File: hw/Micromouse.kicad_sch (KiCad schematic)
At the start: 19 parts, among them J1 MOTOR_LEFT, J2 MOTOR_RIGHT, J3 ENCODER_LEFT, J4 ENCODER_RIGHT, J5 LIDAR_360, SW1 Power Switch, U1 LM2596 - 5V, U2 MP1584EN Buck 3V3, U3 ESP32-C3-DevKitM-1

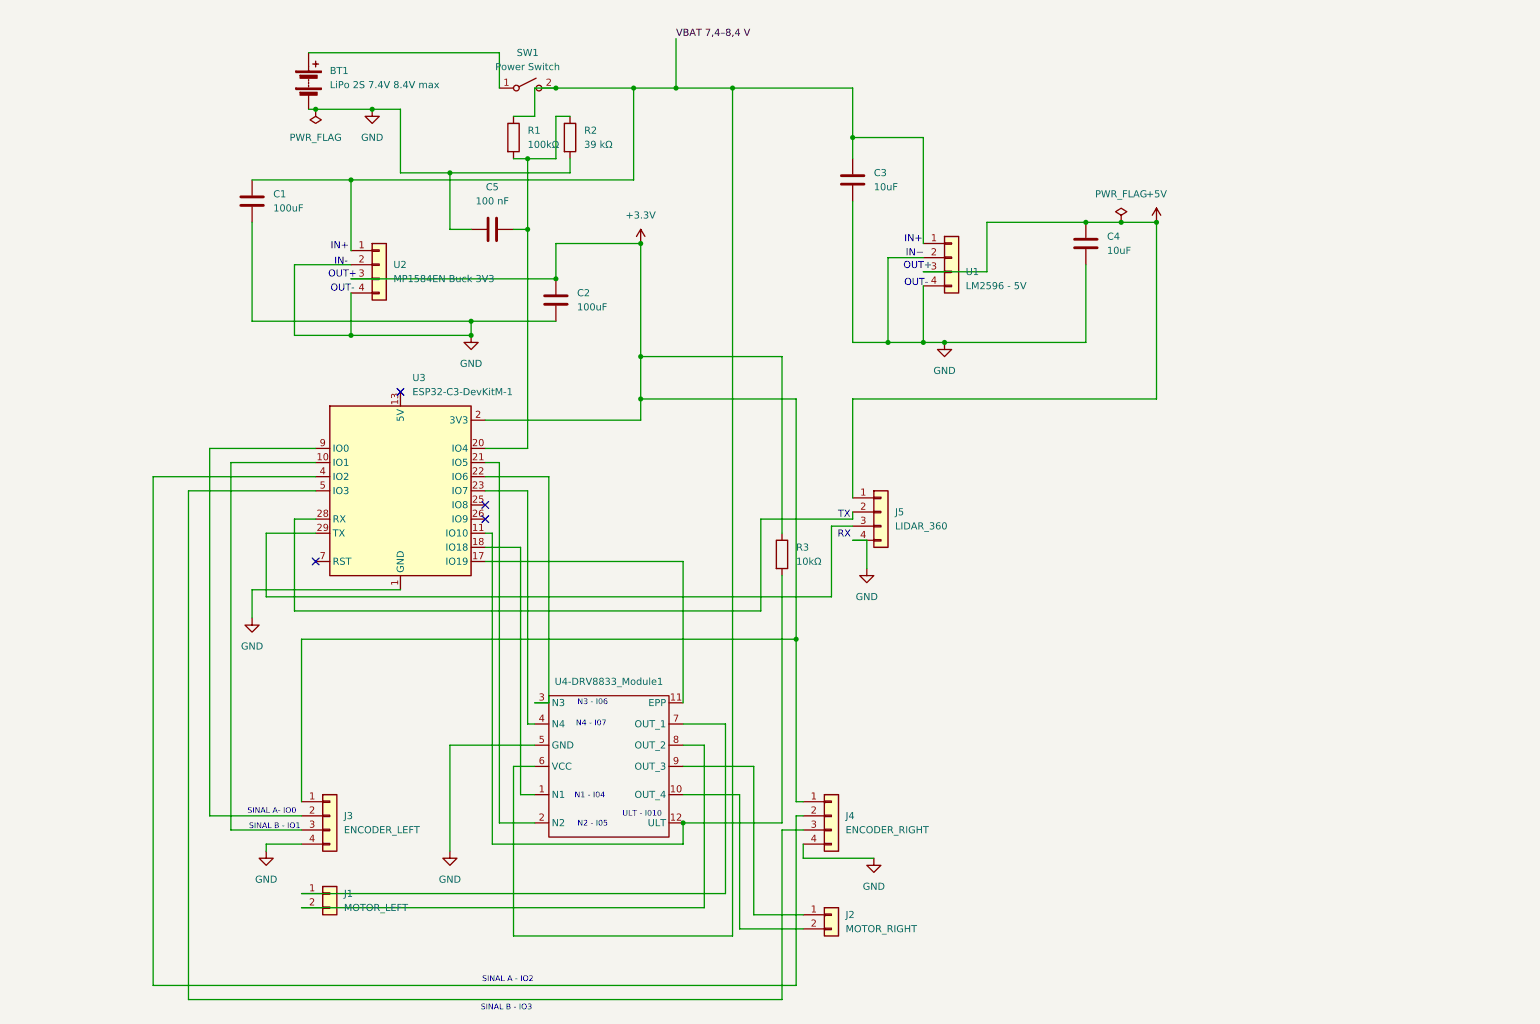
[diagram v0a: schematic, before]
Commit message: feat: atualiza micromouse e kicad
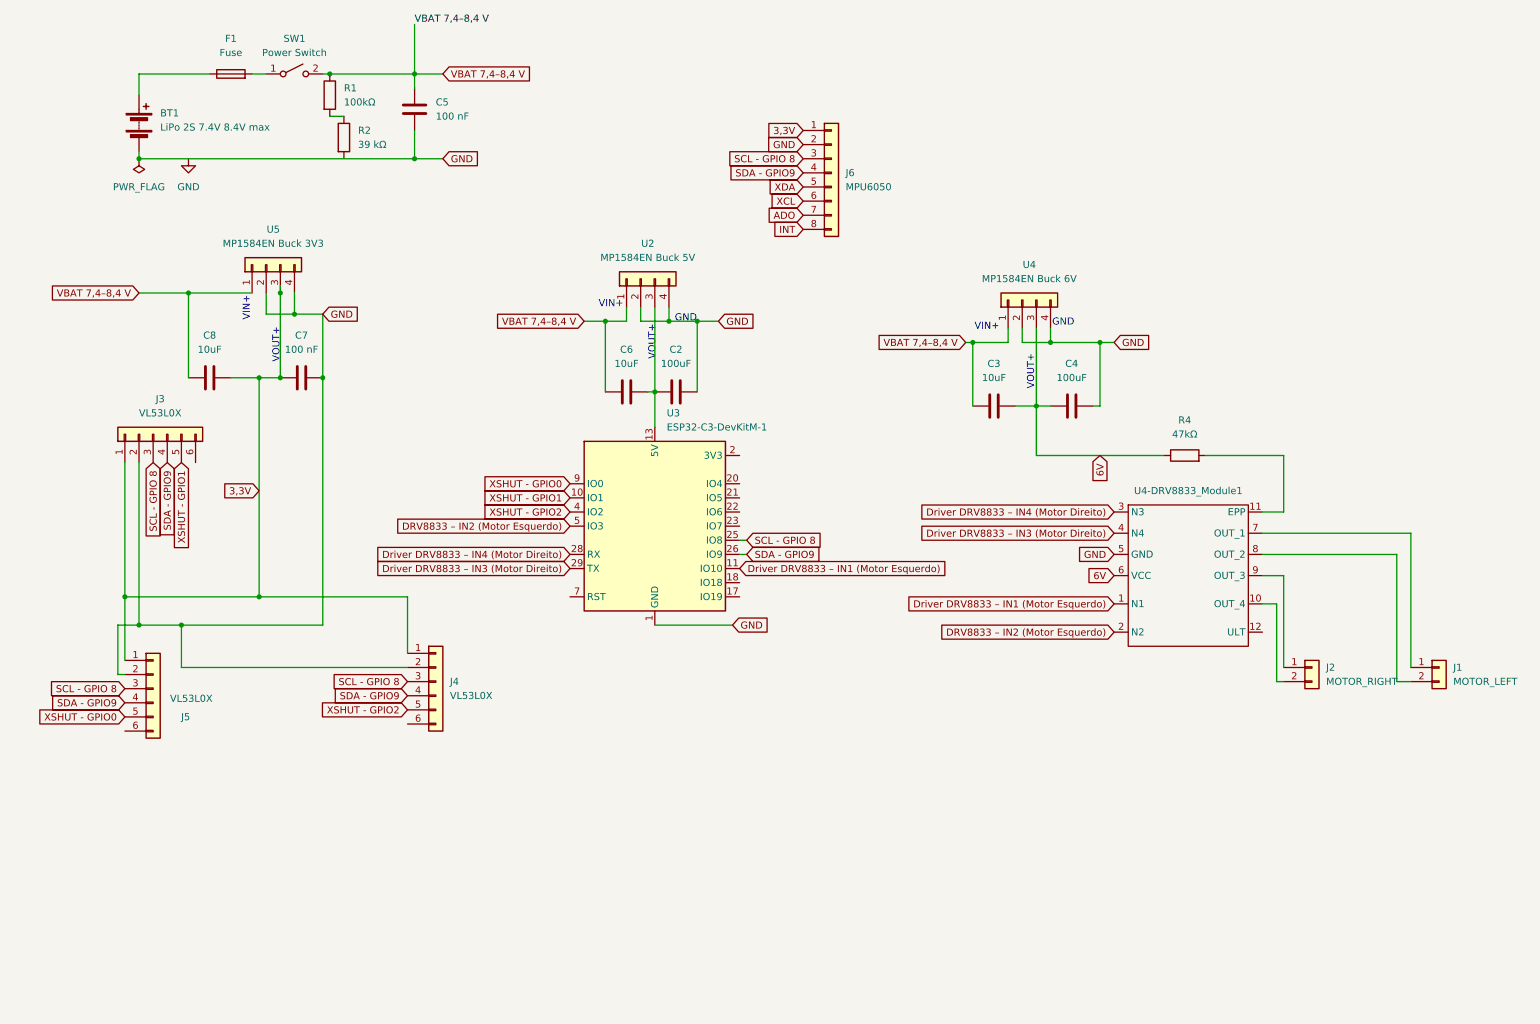
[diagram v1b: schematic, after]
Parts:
- removed C1: 100uF, symbol Device:C
- removed J3: ENCODER_LEFT, Package_TO_SOT_SMD:SOT-223-3_TabPin2, symbol Connector_Generic:Conn_01x04
- removed J4: ENCODER_RIGHT, symbol Connector_Generic:Conn_01x04
- removed J5: LIDAR_360, symbol Connector_Generic:Conn_01x04
- removed R3: 10kΩ, symbol Device:R
- removed U1: LM2596 - 5V, symbol Connector_Generic:Conn_01x04
- added C6, C8: 10uF, symbol Device:C
- added C7: 100 nF, symbol Device:C
- added F1: Fuse, Package_LGA:LGA-28_5.2x3.8mm_P0.5mm, symbol Device:Fuse
- added J3: VL53L0X, Sensor_Distance:ST_VL53L1x, symbol Connector_Generic:Conn_01x06
- added J4, J5: VL53L0X, symbol Connector_Generic:Conn_01x06
- added J6: MPU6050, Package_LCC:PLCC-84_29.3x29.3mm_P1.27mm, symbol Connector_Generic:Conn_01x08
- added R4: 47kΩ, symbol Device:R
- added U4: MP1584EN Buck 6V, Package_TO_SOT_SMD:SOT-223-3_TabPin2, symbol Connector_Generic:Conn_01x04
- added U5: MP1584EN Buck 3V3, Package_TO_SOT_SMD:SOT-223-3_TabPin2, symbol Connector_Generic:Conn_01x04
- C4: value 10uF -> 100uF
- U2: value MP1584EN Buck 3V3 -> MP1584EN Buck 5V
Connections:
- net +5V is gone; now on net GND: C4.1
- net GND: now also C5.2, C7.1, J3.2 (Pin_2), J4.2 (Pin_2), J5.2 (Pin_2), J6.2 (Pin_2), U4.2 (Pin_2), U4.4 (Pin_4), U5.2 (Pin_2), U5.4 (Pin_4); no longer C3.2, C4.2, C5.1, R2.2
- net VBAT  7,4–8,4 V: now also C5.1, C6.1, C8.1, U4.1 (Pin_1), U5.1 (Pin_1); no longer U4-DRV8833_Module1.6 (VCC)
- net Driver DRV8833 – IN4 (Motor Direito): now reaches U3.28 (RX)
- net Driver DRV8833 – IN4 (Motor Direito): now also U4-DRV8833_Module1.3 (N3)
- net Driver DRV8833 – IN3 (Motor Direito): now reaches U3.29 (TX)
- net Driver DRV8833 – IN3 (Motor Direito): now also U4-DRV8833_Module1.4 (N4)
- net at R1.2, R2.1: no longer C5.2, U3.20 (IO4)
- net XSHUT - GPIO2: now reaches U3.4 (IO2)
- net XSHUT - GPIO2: now also J4.5 (Pin_5)
- net DRV8833 – IN2 (Motor Esquerdo): now reaches U3.5 (IO3)
- net DRV8833 – IN2 (Motor Esquerdo): now also U4-DRV8833_Module1.2 (N2)
- net at BT1.1 (+): now also F1.1; no longer SW1.1 (A)
- net XSHUT - GPIO0: now reaches U3.9 (IO0)
- net XSHUT - GPIO0: now also J5.5 (Pin_5)
- net XSHUT - GPIO1: now reaches U3.10 (IO1)
- net XSHUT - GPIO1: now also J3.5 (Pin_5)
- net at U4-DRV8833_Module1.12 (ULT): no longer U3.11 (IO10)
- net at U3.18 (IO18): no longer U4-DRV8833_Module1.1 (N1)
- net at U3.17 (IO19): no longer U4-DRV8833_Module1.11 (EPP)
- net at U3.21 (IO5): no longer U4-DRV8833_Module1.2 (N2)
- net at U3.22 (IO6): no longer U4-DRV8833_Module1.3 (N3)
- net at U3.23 (IO7): no longer U4-DRV8833_Module1.4 (N4)
- net at U3.13 (5V), U3.14 (5V): now also C2.1, U2.3 (Pin_3), C6.2
- net SCL - GPIO 8: now reaches U3.25 (IO8)
- net SCL - GPIO 8: now also J3.3 (Pin_3), J4.3 (Pin_3), J5.3 (Pin_3), J6.3 (Pin_3)
- net SDA - GPIO9: now reaches U3.26 (IO9)
- net SDA - GPIO9: now also J3.4 (Pin_4), J4.4 (Pin_4), J5.4 (Pin_4), J6.4 (Pin_4)
- net +3.3V: no longer names the net of U3.2 (3V3), U3.3 (3V3)
- net +3.3V: no longer C2.1, U2.3 (Pin_3)
- new net: F1.2, SW1.1 (A)
- new net: R4.2, U4-DRV8833_Module1.11 (EPP)
- new net 3,3V: C7.2, C8.2, J3.1 (Pin_1), J4.1 (Pin_1), J5.1 (Pin_1), J6.1 (Pin_1), U5.3 (Pin_3)
- new net 6V: C3.2, C4.2, R4.1, U4-DRV8833_Module1.6 (VCC), U4.3 (Pin_3)
- new net ADO: J6.7 (Pin_7)
- new net Driver DRV8833 – IN1 (Motor Esquerdo): U3.11 (IO10), U4-DRV8833_Module1.1 (N1)
- new net INT: J6.8 (Pin_8)
- new net XCL: J6.6 (Pin_6)
- new net XDA: J6.5 (Pin_5)
- no-connect marks 4 -> 0
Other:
- note added: "GND"
- note added: "VIN+"
- note added: "VOUT+"
- note removed: "IN+"
- note removed: "IN-"
- note removed: "IN−"
- note removed: "N1 - I04"
- note removed: "N2 - I05"
- note removed: "N3 - I06"
- note removed: "N4 - I07"
- note removed: "OUT+"
- note removed: "OUT-"
- note removed: "RX"
- note removed: "SINAL A - IO2"
- note removed: "SINAL A- IO0"
- note removed: "SINAL B - IO1"
- note removed: "SINAL B - IO3"
- note removed: "TX"
- note removed: "ULT - I010"
